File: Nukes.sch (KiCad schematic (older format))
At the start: 30 parts, among them J5 Screw_Terminal_01x02, J6 Screw_Terminal_01x02, J7 Screw_Terminal_01x02, J8 Screw_Terminal_01x02, Q4 PMV20ENR, Q5 PMV20ENR, SW3 SW_DPDT_x2, SW4 SW_DPDT_x2, U10 LTV-817S, U9 LTV-817S

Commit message: Add files via upload
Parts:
- removed D13, D9: ARM, LED_SMD:LED_0603_1608Metric_Castellated, symbol Device:LED
- removed J5: Screw_Terminal_01x02, TerminalBlock_Phoenix:TerminalBlock_Phoenix_MPT-0,5-2-2.54_1x02_P2.54mm_Horizontal, symbol Connector:Screw_Terminal_01x02
- removed R26, R31: 470, Resistor_SMD:R_0603_1608Metric, symbol Device:R
- removed SW3, SW4: SW_DPDT_x2, Button_Switch_THT:SW_CuK_JS202011AQN_DPDT_Angled, symbol Switch:SW_DPDT_x2
- R27, R30, R32, R35: value 470 -> 1k
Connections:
- net labels added: External_Supply
- net labels removed: CONT, Fire
- wire segments 178 -> 145
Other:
- moved on the sheet: D10, D11, D12, D14, D15, D16, J6, J7, J8, JP3, JP4, Q4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

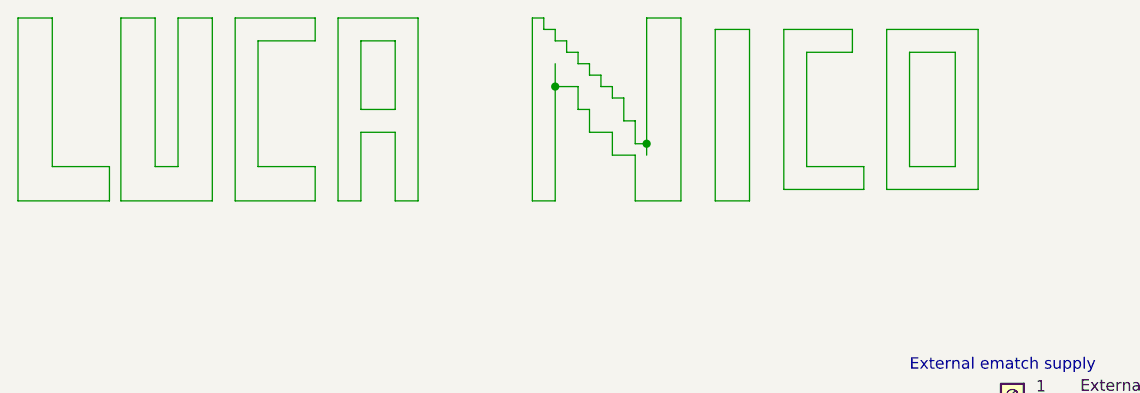
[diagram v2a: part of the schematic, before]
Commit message: Add files via upload
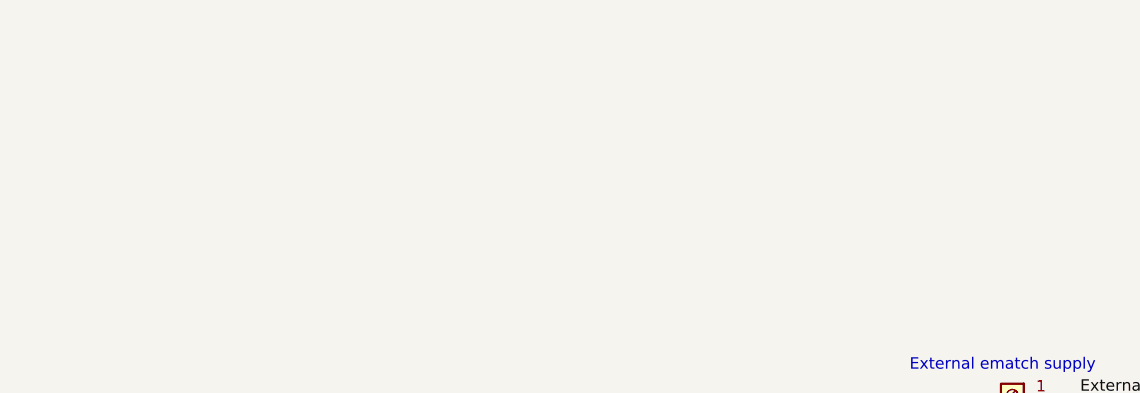
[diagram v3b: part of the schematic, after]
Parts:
- JP3, JP4: footprint Jumper:SolderJumper-3_P1.3mm_Open_RoundedPad1.0x1.5mm_NumberLabels -> Jumper:SolderJumper-3_P2.0mm_Open_TrianglePad1.0x1.5mm_NumberLabels
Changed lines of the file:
@@
 	1    0    0    -1
 $EndComp
-Wire Wire Line
-	900  950  900  1750
-Wire Wire Line
-	900  1750 1300 1750
-Wire Wire Line
-	1300 1750 1300 1600
-Wire Wire Line
-	1300 1600 1050 1600
-Wire Wire Line
-	1050 1600 1050 950
-Wire Wire Line
-	1050 950  900  950
-Wire Wire Line
-	1350 950  1350 1750
-Wire Wire Line
-	1350 1750 1750 1750
-Wire Wire Line
-	1750 1750 1750 950
-Wire Wire Line
-	1750 950  1600 950
-Wire Wire Line
-	1600 950  1600 1600
-Wire Wire Line
-	1600 1600 1500 1600
-Wire Wire Line
-	1500 1600 1500 950
-Wire Wire Line
-	1500 950  1350 950
-Wire Wire Line
-	2200 950  1850 950
-Wire Wire Line
-	1850 950  1850 1750
-Wire Wire Line
-	1850 1750 2200 1750
-Wire Wire Line
-	2200 1750 2200 1600
-Wire Wire Line
-	2200 1600 1950 1600
-Wire Wire Line
-	1950 1600 1950 1050
-Wire Wire Line
-	1950 1050 2200 1050
-Wire Wire Line
-	2200 1050 2200 950
-Wire Wire Line
-	2300 1750 2300 950
-Wire Wire Line
-	2300 950  2650 950
-Wire Wire Line
-	2650 950  2650 1750
-Wire Wire Line
-	2650 1750 2550 1750
-Wire Wire Line
-	2550 1750 2550 1450
-Wire Wire Line
-	2550 1450 2400 1450
-Wire Wire Line
-	2400 1450 2400 1750
-Wire Wire Line
-	2400 1750 2300 1750
-Wire Wire Line
-	2400 1350 2400 1050
-Wire Wire Line
-	2400 1050 2550 1050
-Wire Wire Line
-	2550 1050 2550 1350
-Wire Wire Line
-	2550 1350 2400 1350
-Wire Wire Line
-	3150 1750 3150 950
-Wire Wire Line
-	3150 950  3200 950
-Wire Wire Line
-	3200 950  3200 1000
-Wire Wire Line
-	3200 1000 3250 1000
-Wire Wire Line
-	3250 1000 3250 1050
-Wire Wire Line
-	3250 1050 3300 1050
-Wire Wire Line
-	3300 1050 3300 1100
-Wire Wire Line
-	3300 1100 3350 1100
-Wire Wire Line
-	3350 1100 3350 1150
-Wire Wire Line
-	3350 1150 3400 1150
-Wire Wire Line
-	3400 1150 3400 1200
-Wire Wire Line
-	3400 1200 3450 1200
-Wire Wire Line
-	3450 1200 3450 1250
-Wire Wire Line
-	3450 1250 3500 1250
-Wire Wire Line
-	3500 1250 3500 1300
-Wire Wire Line
-	3500 1300 3550 1300
-Wire Wire Line
-	3550 1300 3550 1400
-Wire Wire Line
-	3550 1400 3600 1400
-Wire Wire Line
-	3600 1400 3600 1500
-Wire Wire Line
-	3600 1500 3650 1500
-Wire Wire Line
-	3650 950  3800 950
-Wire Wire Line
-	3800 1750 3600 1750
-Wire Wire Line
-	3600 1750 3600 1550
-Wire Wire Line
-	3600 1550 3500 1550
-Wire Wire Line
-	3500 1550 3500 1450
-Wire Wire Line
-	3500 1450 3400 1450
-Wire Wire Line
-	3400 1450 3400 1350
-Wire Wire Line
-	3400 1350 3350 1350
-Wire Wire Line
-	3350 1350 3350 1250
-Wire Wire Line
-	3350 1250 3250 1250
-Wire Wire Line
-	3650 950  3650 1500
-Wire Wire Line
-	3800 950  3800 1750
-Wire Wire Line
-	3250 1150 3250 1250
-Connection ~ 3650 1500
-Wire Wire Line
-	3650 1500 3650 1550
-Connection ~ 3250 1250
-Wire Wire Line
-	3250 1250 3250 1750
-Wire Wire Line
-	3950 1000 3950 1750
-Wire Wire Line
-	3950 1750 4100 1750
-Wire Wire Line
-	4100 1750 4100 1000
-Wire Wire Line
-	4100 1000 3950 1000
-Wire Wire Line
-	4550 1000 4250 1000
-Wire Wire Line
-	4250 1000 4250 1700
-Wire Wire Line
-	4250 1700 4600 1700
-Wire Wire Line
-	4600 1700 4600 1600
-Wire Wire Line
-	4600 1600 4350 1600
-Wire Wire Line
-	4350 1600 4350 1100
-Wire Wire Line
-	4350 1100 4550 1100
-Wire Wire Line
-	4550 1100 4550 1000
-Wire Wire Line
-	4700 1000 5100 1000
-Wire Wire Line
-	5100 1000 5100 1700
-Wire Wire Line
-	5100 1700 4700 1700
-Wire Wire Line
-	4700 1700 4700 1000
-Wire Wire Line
-	4800 1100 5000 1100
-Wire Wire Line
-	5000 1100 5000 1600
-Wire Wire Line
-	5000 1600 4800 1600
-Wire Wire Line
-	4800 1600 4800 1100
-Wire Wire Line
-	3150 1750 3250 1750
 $Comp
 L Connector:Screw_Terminal_01x02 J?
@@
 F 0 "JP4" H 7550 4005 50  0000 C CNN
 F 1 "SolderJumper_3_Open" H 7550 3914 50  0000 C CNN
-F 2 "Jumper:SolderJumper-3_P1.3mm_Open_RoundedPad1.0x1.5mm_NumberLabels" H 7550 3800 50  0001 C CNN
+F 2 "Jumper:SolderJumper-3_P2.0mm_Open_TrianglePad1.0x1.5mm_NumberLabels" H 7550 3800 50  0001 C CNN
 F 3 "~" H 7550 3800 50  0001 C CNN
 	1    7550 3800
@@
 F 0 "JP3" H 3250 4155 50  0000 C CNN
 F 1 "SolderJumper_3_Open" H 3250 4064 50  0000 C CNN
-F 2 "Jumper:SolderJumper-3_P1.3mm_Open_RoundedPad1.0x1.5mm_NumberLabels" H 3250 3950 50  0001 C CNN
+F 2 "Jumper:SolderJumper-3_P2.0mm_Open_TrianglePad1.0x1.5mm_NumberLabels" H 3250 3950 50  0001 C CNN
 F 3 "~" H 3250 3950 50  0001 C CNN
 	1    3250 3950
